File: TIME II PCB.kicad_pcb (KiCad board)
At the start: 2 copper layers, 62 parts, among them J1 SD_Card, J2 USB_C_Receptacle, J3 Conn_01x06, J4 Conn_01x06, J5 Conn_01x06, J6 Conn_01x02_Male, J7 Conn_01x02_Male, J8 Conn_01x02_Pin, Q1 VNP10N07, Q2 VNP10N07, Q3 VNP10N07, SW1 SW_SPDT, U1 STM32F103C8Tx, U2 LTC4420CMSE-PBF, Y1 16 khz

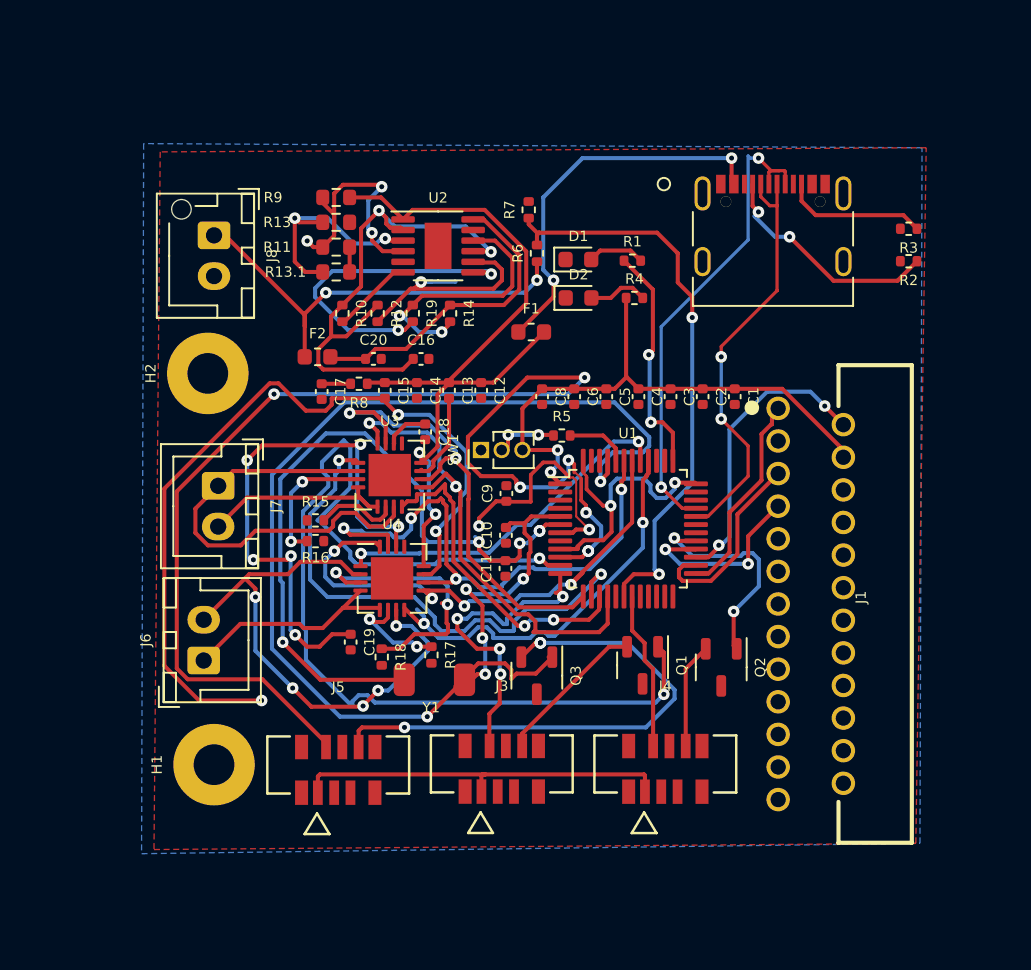
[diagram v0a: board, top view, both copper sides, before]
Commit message: major reroute
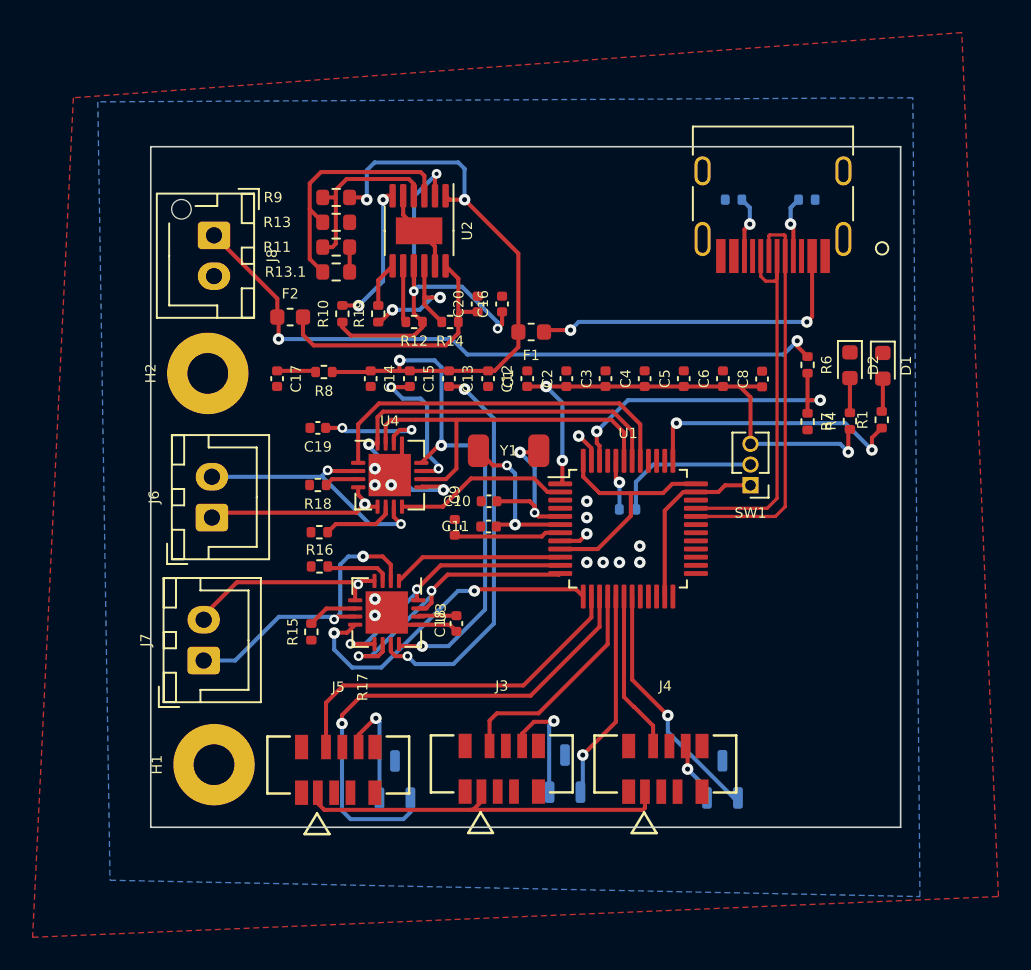
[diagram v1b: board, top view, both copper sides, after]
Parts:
- removed J1: SD_Card, sdcardd:HZIP25-P-1
- Q1, Q2, Q3, R2, R3, R5: moved to B.Cu
- moved R7 21.5 mm to (124.0, 52.6), turned to -90 degrees
- moved D1 19.8 mm to (128.7, 49.2), turned to -90 degrees
- moved R1 18.1 mm to (128.6, 52.5), turned to 90 degrees
- moved R6 18.0 mm to (124.0, 49.1), turned to -90 degrees
- moved D2 17.2 mm to (126.6, 49.2), turned to -90 degrees
- moved SW1 16.7 mm to (120.5, 56.5), turned to 180 degrees
- moved R4 15.2 mm to (126.6, 52.6), turned to 90 degrees
- moved Y1 14.8 mm to (105.7, 54.4)
- moved C8 13.5 mm to (121.2, 50.0), turned to 90 degrees
- moved C19 13.3 mm to (94.0, 53.0), turned to 180 degrees
- moved C1 12.8 mm to (106.8, 50.0), turned to 90 degrees
- moved C18 11.9 mm to (102.5, 65.0)
- moved R18 11.3 mm to (94.0, 56.5), turned to 180 degrees
- moved R3 10.9 mm to (119.5, 39.0)
- moved Q3 10.8 mm to (98.7, 74.6), turned to 90 degrees
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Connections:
- U1 pad 10: therm_2 -> MOT_CON2
- U1 pad 11: heater_1 -> SERVO_2
- U1 pad 12: therm_1 -> SERVO_2A
- U1 pad 13: SERVO_2A -> MOT_MON_2
- U1 pad 14: MOT_CON2 -> therm_2
- U1 pad 15: MOT_MON_2 -> heater_2
- U1 pad 16: SERVO_2 -> therm_1
- U1 pad 17: unconnected-(U1-PA7-Pad17) -> heater_1
- U1 pad 18: V_MON -> therm_3
- U1 pad 19: therm_3 -> heater_3
- U1 pad 2: unconnected-(U1-PC13-Pad2) -> MOT_MON_1
- U1 pad 29: heater_3 -> unconnected-(U1-PA8-Pad29)
- U1 pad 40: MOT_MON_1 -> unconnected-(U1-PB4-Pad40)
- U1 pad 45: heater_2 -> unconnected-(U1-PB8-Pad45)
- U1 pad 46: unconnected-(U1-PB9-Pad46) -> V_MON
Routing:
- net therm_2: track 77.2 -> 22.5 mm, vias 7 -> 0
- net heater_1: track 64.7 -> 12.9 mm, vias 2 -> 1
- net Net-(U4-VCP): track 50.8 -> 9.12 mm, vias 3 -> 2
- net heater_2: track 64.9 -> 31.2 mm, vias 2 -> 1
- net Net-(U1-PD1): track 43.7 -> 10.2 mm, vias 5 -> 2
- net GND: track 0.03 -> 27.0 mm, vias 0 -> 14
- net Net-(U4-VINT): track 33.7 -> 7.09 mm, vias 6 -> 2
- net Net-(J5-Pin_6): track 32.7 -> 7.28 mm, vias 3 -> 1
- net MOT_CON2: track 32.7 -> 10.5 mm, vias 2 -> 0
- net Net-(U3-VCP): track 5.52 -> 24.3 mm, vias 0 -> 2
- net MISO: track 18.1 -> 0.00 mm, vias 2 -> 0
- net Net-(U2-GNDSW): track 20.1 -> 2.79 mm, vias 2 -> 0
- net MOTOR_1: track 33.4 -> 17.0 mm, vias 5 -> 2
- net V_MON: track 35.4 -> 19.6 mm
- net USB_P: track 49.0 -> 63.8 mm, vias 2 -> 5
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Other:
- board outline added: 46 x 41.8 mm
